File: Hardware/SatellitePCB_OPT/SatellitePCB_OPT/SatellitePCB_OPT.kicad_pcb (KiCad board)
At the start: 4 copper layers, 61 x 61 mm, 15 parts, among them IC1 OPT3001DNPRQ1, IC2 OPT3001DNPRQ1, IC3 OPT3001DNPRQ1, IC4 OPT3001DNPRQ1, J2 SM08B-SRSS-TB_LF__SN_

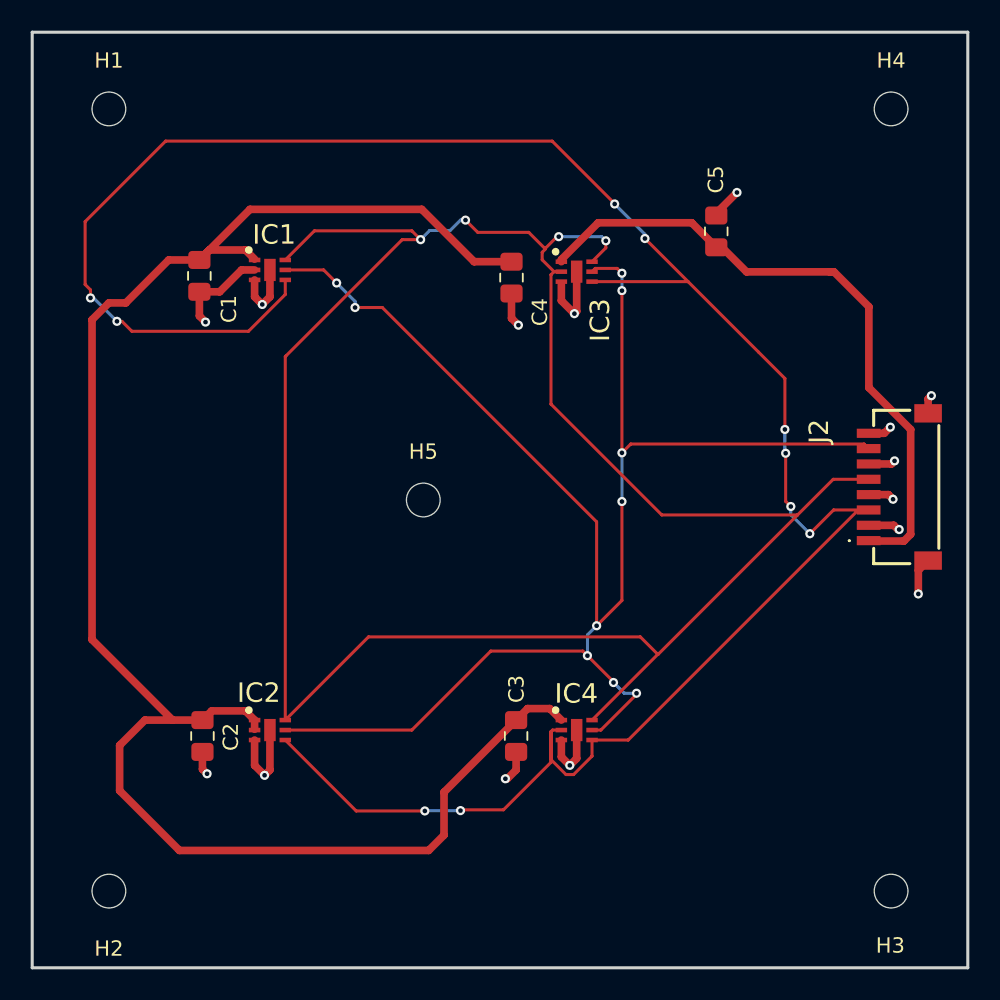
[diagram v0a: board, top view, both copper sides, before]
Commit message: cambios menores
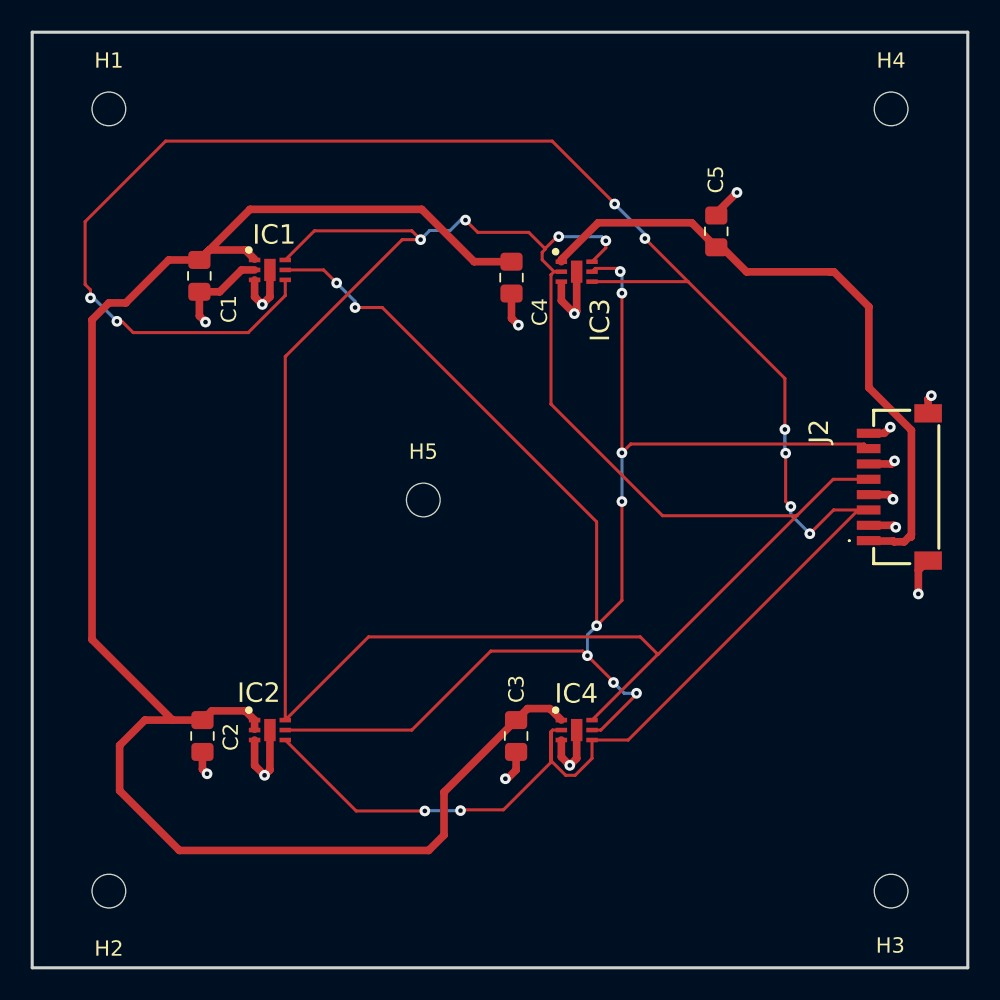
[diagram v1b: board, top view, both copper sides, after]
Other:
- copper layers 4 -> 2
